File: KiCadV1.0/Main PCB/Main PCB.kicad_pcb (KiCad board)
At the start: 2 copper layers, 6 parts, among them J1 Conn_01x01_Male, J2 Conn_01x01_Male, U1 TM1637, U2 TM1637, U3 TM1637

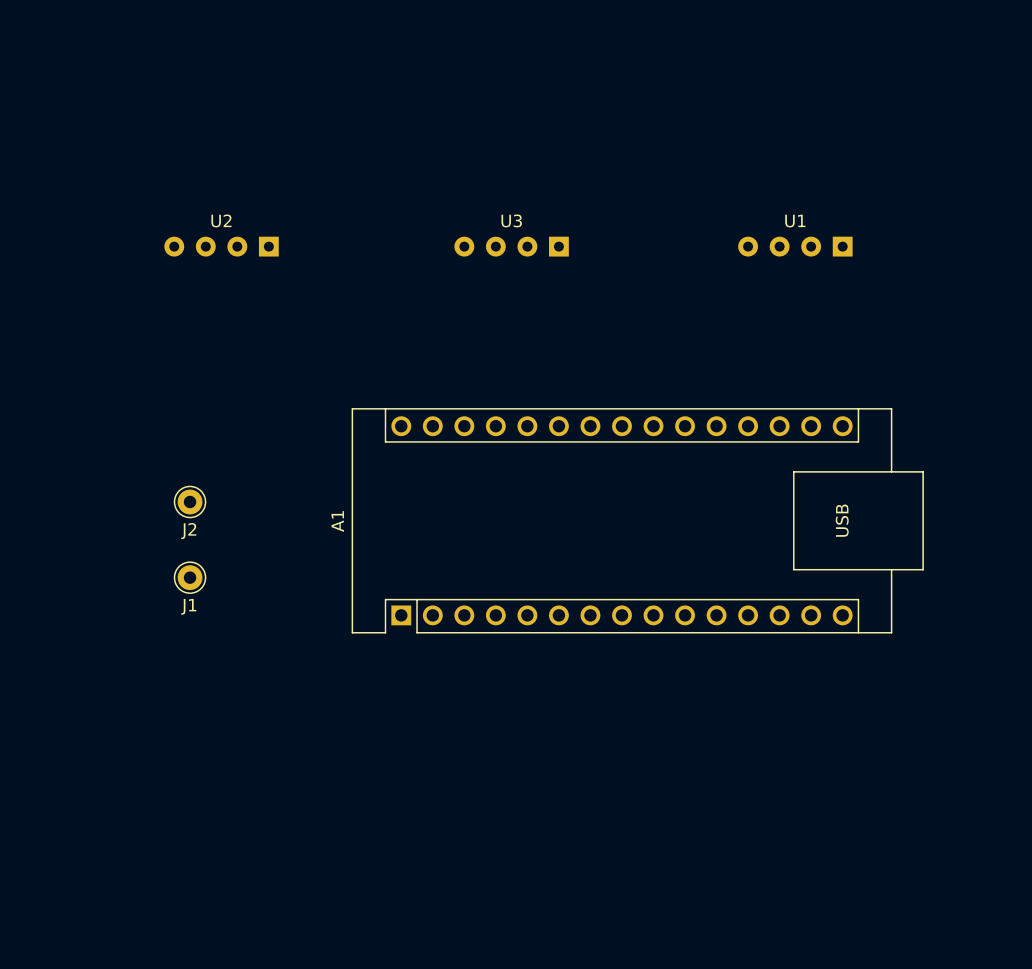
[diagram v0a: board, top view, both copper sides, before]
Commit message: PCB terminé
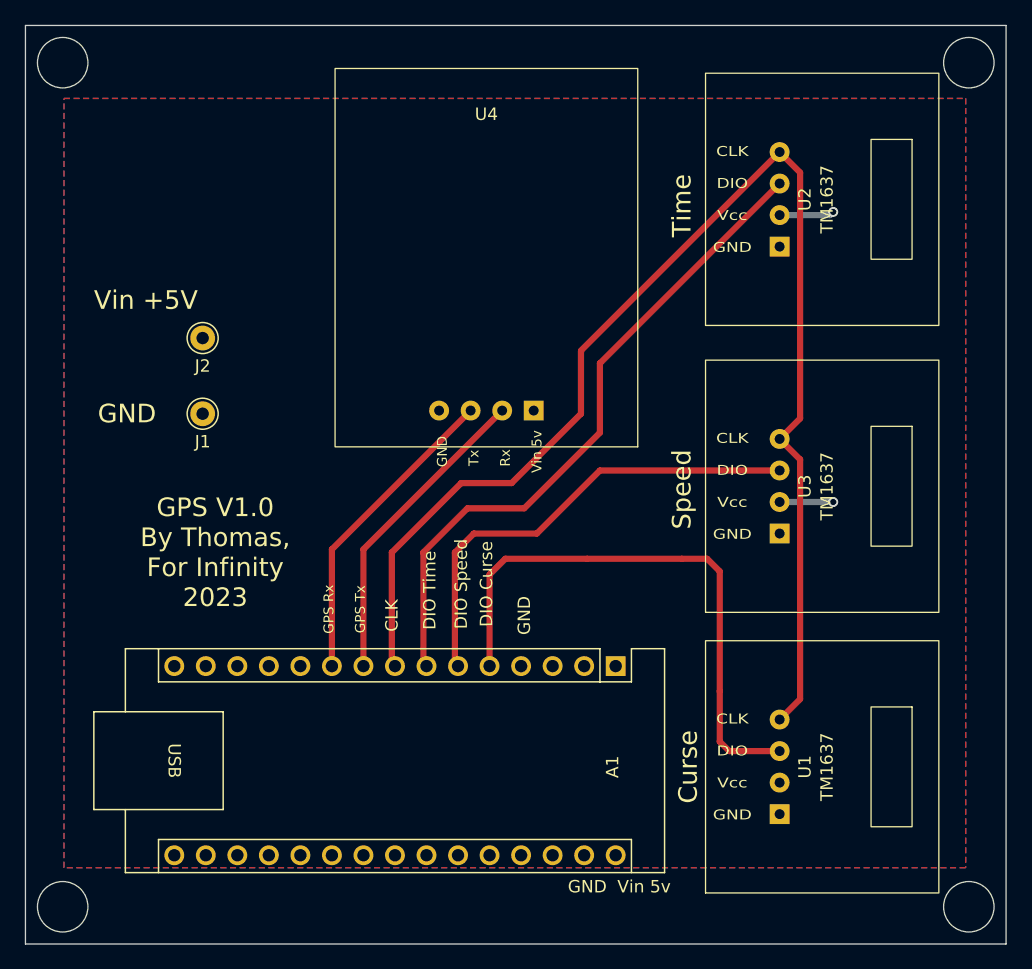
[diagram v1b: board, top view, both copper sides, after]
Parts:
- added U4: NEO6M, thomas footprint:NEO6M, F.Cu at (72.1, 78.2)
- U1, U2, U3: footprint thomas:TM1637 -> thomas footprint:TM1637
- moved U2 47.8 mm to (98.6, 64.0), turned to -90 degrees
- moved U1 44.7 mm to (98.6, 109.7), turned to -90 degrees
- moved U3 32.9 mm to (98.6, 87.1), turned to -90 degrees
- moved A1 17.7 mm to (82.5, 101.6), turned to -90 degrees
- moved J1 13.2 mm to (49.3, 81.3)
- moved J2 13.2 mm to (49.3, 75.2)
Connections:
- A1 pad 10: unconnected-(A1-Pad10) -> Net-(U4-Pad3)
- A1 pad 13: Net-(A1-Pad13) -> unconnected-(A1-Pad13)
- A1 pad 14: Net-(A1-Pad14) -> unconnected-(A1-Pad14)
- A1 pad 15: Net-(A1-Pad15) -> unconnected-(A1-Pad15)
- A1 pad 16: Net-(A1-Pad16) -> unconnected-(A1-Pad16)
- A1 pad 29: unconnected-(A1-Pad29) -> GND
- A1 pad 4: unconnected-(A1-Pad4) -> GND
- A1 pad 5: unconnected-(A1-Pad5) -> Net-(U1-Pad3)
- A1 pad 6: unconnected-(A1-Pad6) -> Net-(A1-Pad6)
- A1 pad 7: unconnected-(A1-Pad7) -> Net-(A1-Pad7)
- A1 pad 8: unconnected-(A1-Pad8) -> Net-(U1-Pad4)
- A1 pad 9: unconnected-(A1-Pad9) -> Net-(U4-Pad2)
- U1 pad 3: Net-(A1-Pad16) -> Net-(U1-Pad3)
- U1 pad 4: Net-(A1-Pad13) -> Net-(U1-Pad4)
- U2 pad 3: Net-(A1-Pad15) -> Net-(A1-Pad7)
- U2 pad 4: Net-(A1-Pad13) -> Net-(U1-Pad4)
- U3 pad 3: Net-(A1-Pad14) -> Net-(A1-Pad6)
- U3 pad 4: Net-(A1-Pad13) -> Net-(U1-Pad4)
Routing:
- net Net-(U1-Pad4): track 0.00 -> 105.3 mm
- net Net-(A1-Pad7): track 0.00 -> 53.5 mm
- net Net-(U1-Pad3): track 0.00 -> 45.7 mm
- net Net-(A1-Pad6): track 0.00 -> 38.2 mm
- net Net-(U4-Pad2): track 0.00 -> 25.2 mm
- net Net-(U4-Pad3): track 0.00 -> 25.2 mm
- net Vin5v: track 0.00 -> 8.74 mm, vias 0 -> 2
- added copper zone on B.Cu, net GND
- added copper zone on F.Cu, net Vin5v
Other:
- board outline added: 79 x 74 mm
- board text added: "CLK"
- board text added: "CLK DIO Vcc GND"
- board text added: "Curse"
- board text added: "DIO Curse"
- board text added: "DIO Speed"
- board text added: "DIO Time"
- board text added: "GND"
- board text added: "GPS Rx"
- board text added: "GPS Tx"
- board text added: "GPS V1.0 By Thomas, For Infinity 2023"
- board text added: "Rx"
- board text added: "Speed"
- board text added: "Time"
- board text added: "Tx"
- board text added: "Vin +5V"
- board text added: "Vin 5v"
